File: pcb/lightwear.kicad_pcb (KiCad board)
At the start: 2 copper layers, 55 x 20 mm, 40 parts, among them J1 USB_C_Receptacle_USB2.0_16P, Q1 PMOS, SW1 SW_SPST, U1 LT1618EDD-PBF, U2 MCP73831-2-OT, U3 ATtiny1616-M

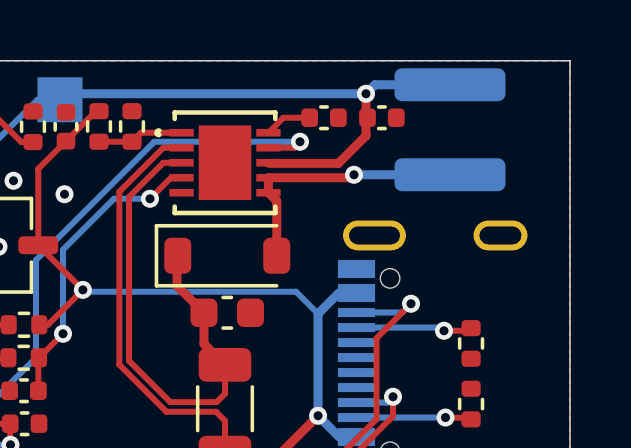
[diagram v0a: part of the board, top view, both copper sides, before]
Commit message: small tweak
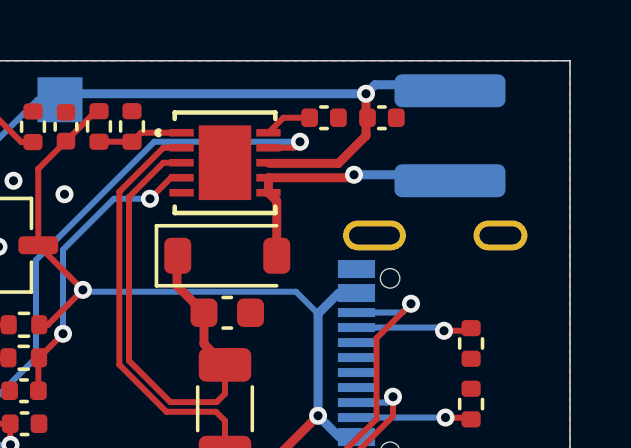
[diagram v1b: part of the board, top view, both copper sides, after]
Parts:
- moved L1 0.20 mm to (173.0, 55.5)
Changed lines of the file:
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@@
 	(footprint "Inductor_SMD:L_Changjiang_FNR4030S"
 		(layer "B.Cu")
-		(at 173 55.3 90)
+		(at 173 55.5 90)
 		(descr "Inductor, Changjiang, FNR4030S, 4.0x4.0x3.0mm, (https://datasheet.lcsc.com/lcsc/1806131217_cjiang-Changjiang-Microelectronics-Tech-FNR5040S3R3NT_C167960.pdf), generated with kicad-footprint-generator gen_inductor.py")
 		(tags "wirewound power shielded")
